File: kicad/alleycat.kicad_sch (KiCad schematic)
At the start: 84 parts, among them U1 E73-2G4M08S1C

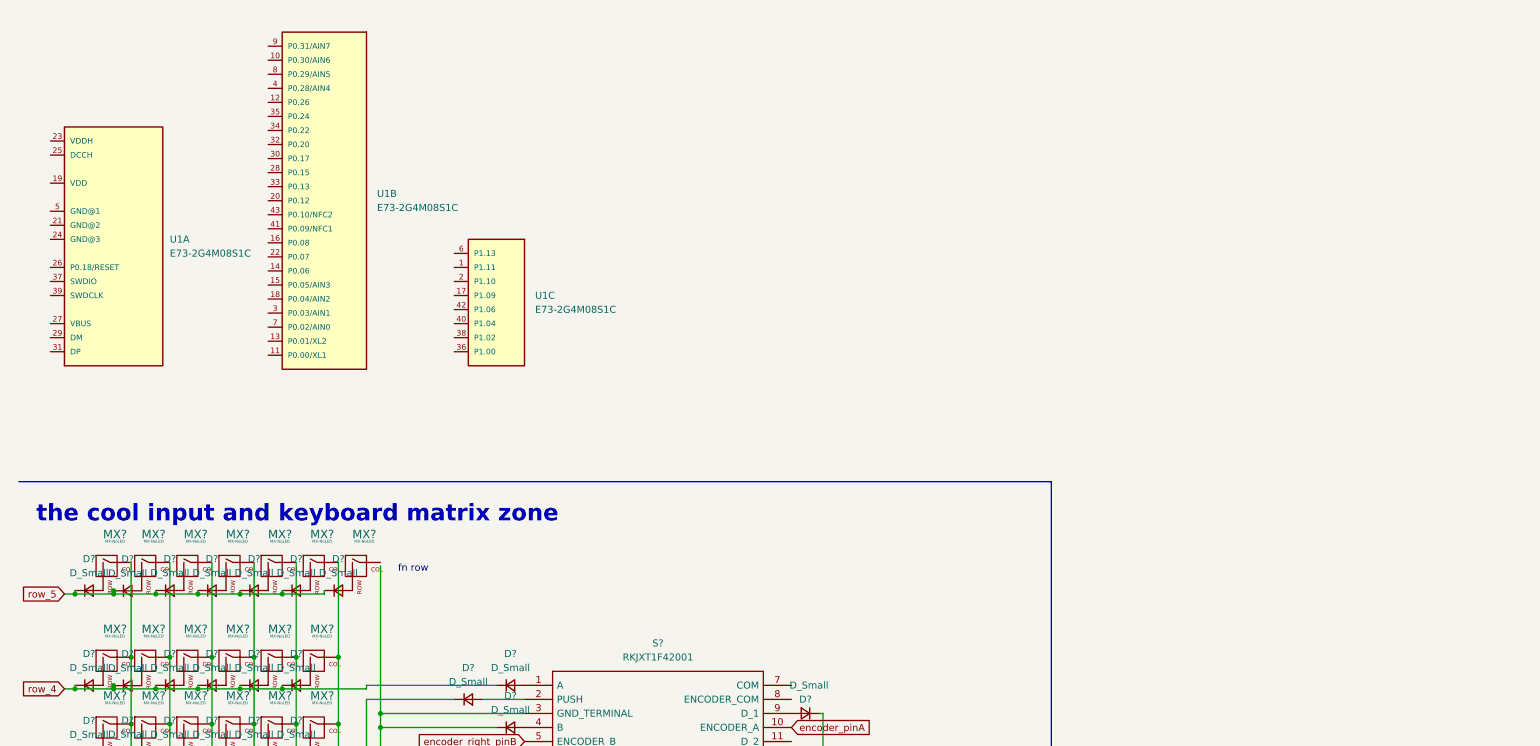
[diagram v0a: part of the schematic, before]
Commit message: nya
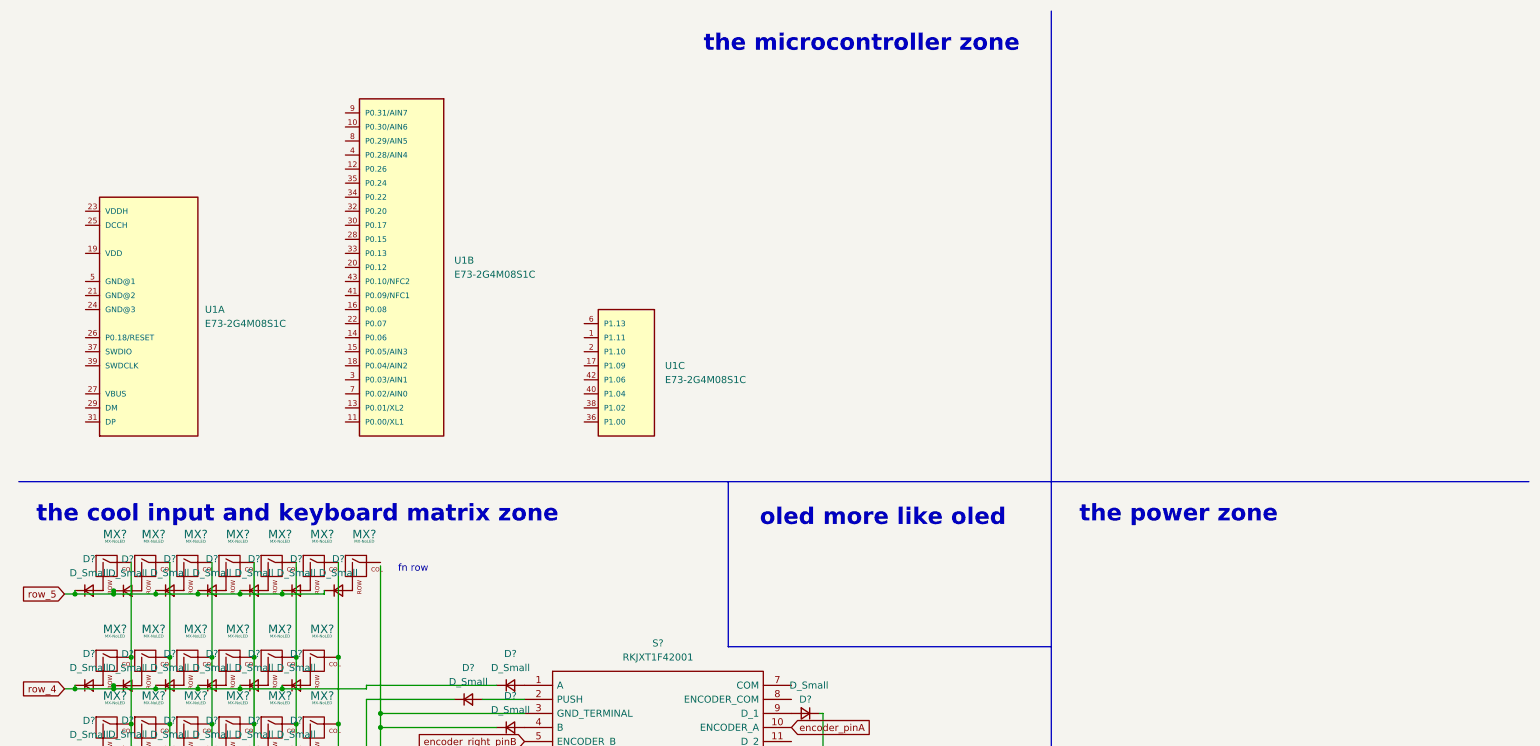
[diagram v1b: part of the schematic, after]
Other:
- note added: "oled more like oled"
- note added: "the microcontroller zone"
- note added: "the power zone"
- moved on the sheet: U1A, U1B, U1C
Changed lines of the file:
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@@
+    (stroke (width 0) (type default) (color 0 0 0 0))
+  )
+  (polyline (pts (xy 140.335 127) (xy 198.755 127))
     (stroke (width 0) (type default) (color 0 0 0 0))
   )
@@
     (stroke (width 0) (type default) (color 0 0 0 0))
   )
+  (polyline (pts (xy 140.335 97.155) (xy 140.335 127))
+    (stroke (width 0) (type default) (color 0 0 0 0))
+  )
   (wire (pts (xy 44.45 146.685) (xy 52.07 146.685))
     (stroke (width 0) (type default) (color 0 0 0 0))
@@
     (stroke (width 0) (type default) (color 0 0 0 0))
   )
+  (polyline (pts (xy 198.755 12.065) (xy 198.755 97.155))
+    (stroke (width 0) (type default) (color 0 0 0 0))
+  )
   (wire (pts (xy 90.805 136.525) (xy 74.93 136.525))
     (stroke (width 0) (type default) (color 0 0 0 0))
@@
   (wire (pts (xy 52.07 184.15) (xy 59.69 184.15))
     (stroke (width 0) (type default) (color 0 0 0 0))
+  )
+  (polyline (pts (xy 198.755 97.155) (xy 285.115 97.155))
+    (stroke (width 0) (type default) (color 0 0 0 0))
+  )
+  (text "the microcontroller zone\n" (at 135.89 19.685 0)
+    (effects (font (size 3 3) bold) (justify left bottom))
   )
   (text "hate that i need another col for one single button"
@@
     (effects (font (size 1.27 1.27)) (justify left bottom))
   )
+  (text "oled more like oled\n" (at 146.05 105.41 0)
+    (effects (font (size 3 3) bold) (justify left bottom))
+  )
   (text "fn row" (at 80.645 113.665 0)
     (effects (font (size 1.27 1.27)) (justify left bottom))
+  )
+  (text "the power zone" (at 203.835 104.775 0)
+    (effects (font (size 3 3) bold) (justify left bottom))
   )
   (text "with the circle pad facing up and flat on the board, pin 4 is left"
@@
     (pin "2")
   )
-  (symbol (lib_id "E73-2G4M08S1C:E73-2G4M08S1C") (at 100.965 66.04 180) (unit 3)
-    (in_bom yes) (on_board yes) (fields_autoplaced)
-    (property "Reference" "U1" (id 0) (at 105.41 63.4999 0)
+  (symbol (lib_id "E73-2G4M08S1C:E73-2G4M08S1C") (at 124.46 78.74 180) (unit 3)
+    (in_bom yes) (on_board yes) (fields_autoplaced)
+    (property "Reference" "U1" (id 0) (at 128.905 76.1999 0)
       (effects (font (size 1.27 1.27)) (justify right))
     )
-    (property "Value" "E73-2G4M08S1C" (id 1) (at 105.41 66.0399 0)
+    (property "Value" "E73-2G4M08S1C" (id 1) (at 128.905 78.7399 0)
       (effects (font (size 1.27 1.27)) (justify right))
     )
-    (property "Footprint" "E73-2G4M08S1C" (id 2) (at 100.965 66.04 0)
+    (property "Footprint" "E73-2G4M08S1C" (id 2) (at 124.46 78.74 0)
       (effects (font (size 1.27 1.27)) (justify left bottom) hide)
     )
-    (property "Datasheet" "" (id 3) (at 100.965 66.04 0)
+    (property "Datasheet" "" (id 3) (at 124.46 78.74 0)
       (effects (font (size 1.27 1.27)) (justify left bottom) hide)
     )
@@
     (pin "2")
   )
-  (symbol (lib_id "E73-2G4M08S1C:E73-2G4M08S1C") (at 69.85 46.355 180) (unit 2)
-    (in_bom yes) (on_board yes) (fields_autoplaced)
-    (property "Reference" "U1" (id 0) (at 76.835 45.0849 0)
+  (symbol (lib_id "E73-2G4M08S1C:E73-2G4M08S1C") (at 83.82 58.42 180) (unit 2)
+    (in_bom yes) (on_board yes) (fields_autoplaced)
+    (property "Reference" "U1" (id 0) (at 90.805 57.1499 0)
       (effects (font (size 1.27 1.27)) (justify right))
     )
-    (property "Value" "E73-2G4M08S1C" (id 1) (at 76.835 47.6249 0)
+    (property "Value" "E73-2G4M08S1C" (id 1) (at 90.805 59.6899 0)
       (effects (font (size 1.27 1.27)) (justify right))
     )
-    (property "Footprint" "E73-2G4M08S1C" (id 2) (at 69.85 46.355 0)
+    (property "Footprint" "E73-2G4M08S1C" (id 2) (at 83.82 58.42 0)
       (effects (font (size 1.27 1.27)) (justify left bottom) hide)
     )
-    (property "Datasheet" "" (id 3) (at 69.85 46.355 0)
+    (property "Datasheet" "" (id 3) (at 83.82 58.42 0)
       (effects (font (size 1.27 1.27)) (justify left bottom) hide)
     )
@@
     (pin "2")
   )
-  (symbol (lib_id "E73-2G4M08S1C:E73-2G4M08S1C") (at 35.56 53.34 0) (unit 1)
-    (in_bom yes) (on_board yes) (fields_autoplaced)
-    (property "Reference" "U1" (id 0) (at 39.37 53.3399 0)
+  (symbol (lib_id "E73-2G4M08S1C:E73-2G4M08S1C") (at 41.91 66.04 0) (unit 1)
+    (in_bom yes) (on_board yes) (fields_autoplaced)
+    (property "Reference" "U1" (id 0) (at 45.72 66.0399 0)
       (effects (font (size 1.27 1.27)) (justify left))
     )
-    (property "Value" "E73-2G4M08S1C" (id 1) (at 39.37 55.8799 0)
+    (property "Value" "E73-2G4M08S1C" (id 1) (at 45.72 68.5799 0)
       (effects (font (size 1.27 1.27)) (justify left))
     )
-    (property "Footprint" "E73-2G4M08S1C" (id 2) (at 35.56 53.34 0)
+    (property "Footprint" "E73-2G4M08S1C" (id 2) (at 41.91 66.04 0)
       (effects (font (size 1.27 1.27)) (justify left bottom) hide)
     )
-    (property "Datasheet" "" (id 3) (at 35.56 53.34 0)
+    (property "Datasheet" "" (id 3) (at 41.91 66.04 0)
       (effects (font (size 1.27 1.27)) (justify left bottom) hide)
     )

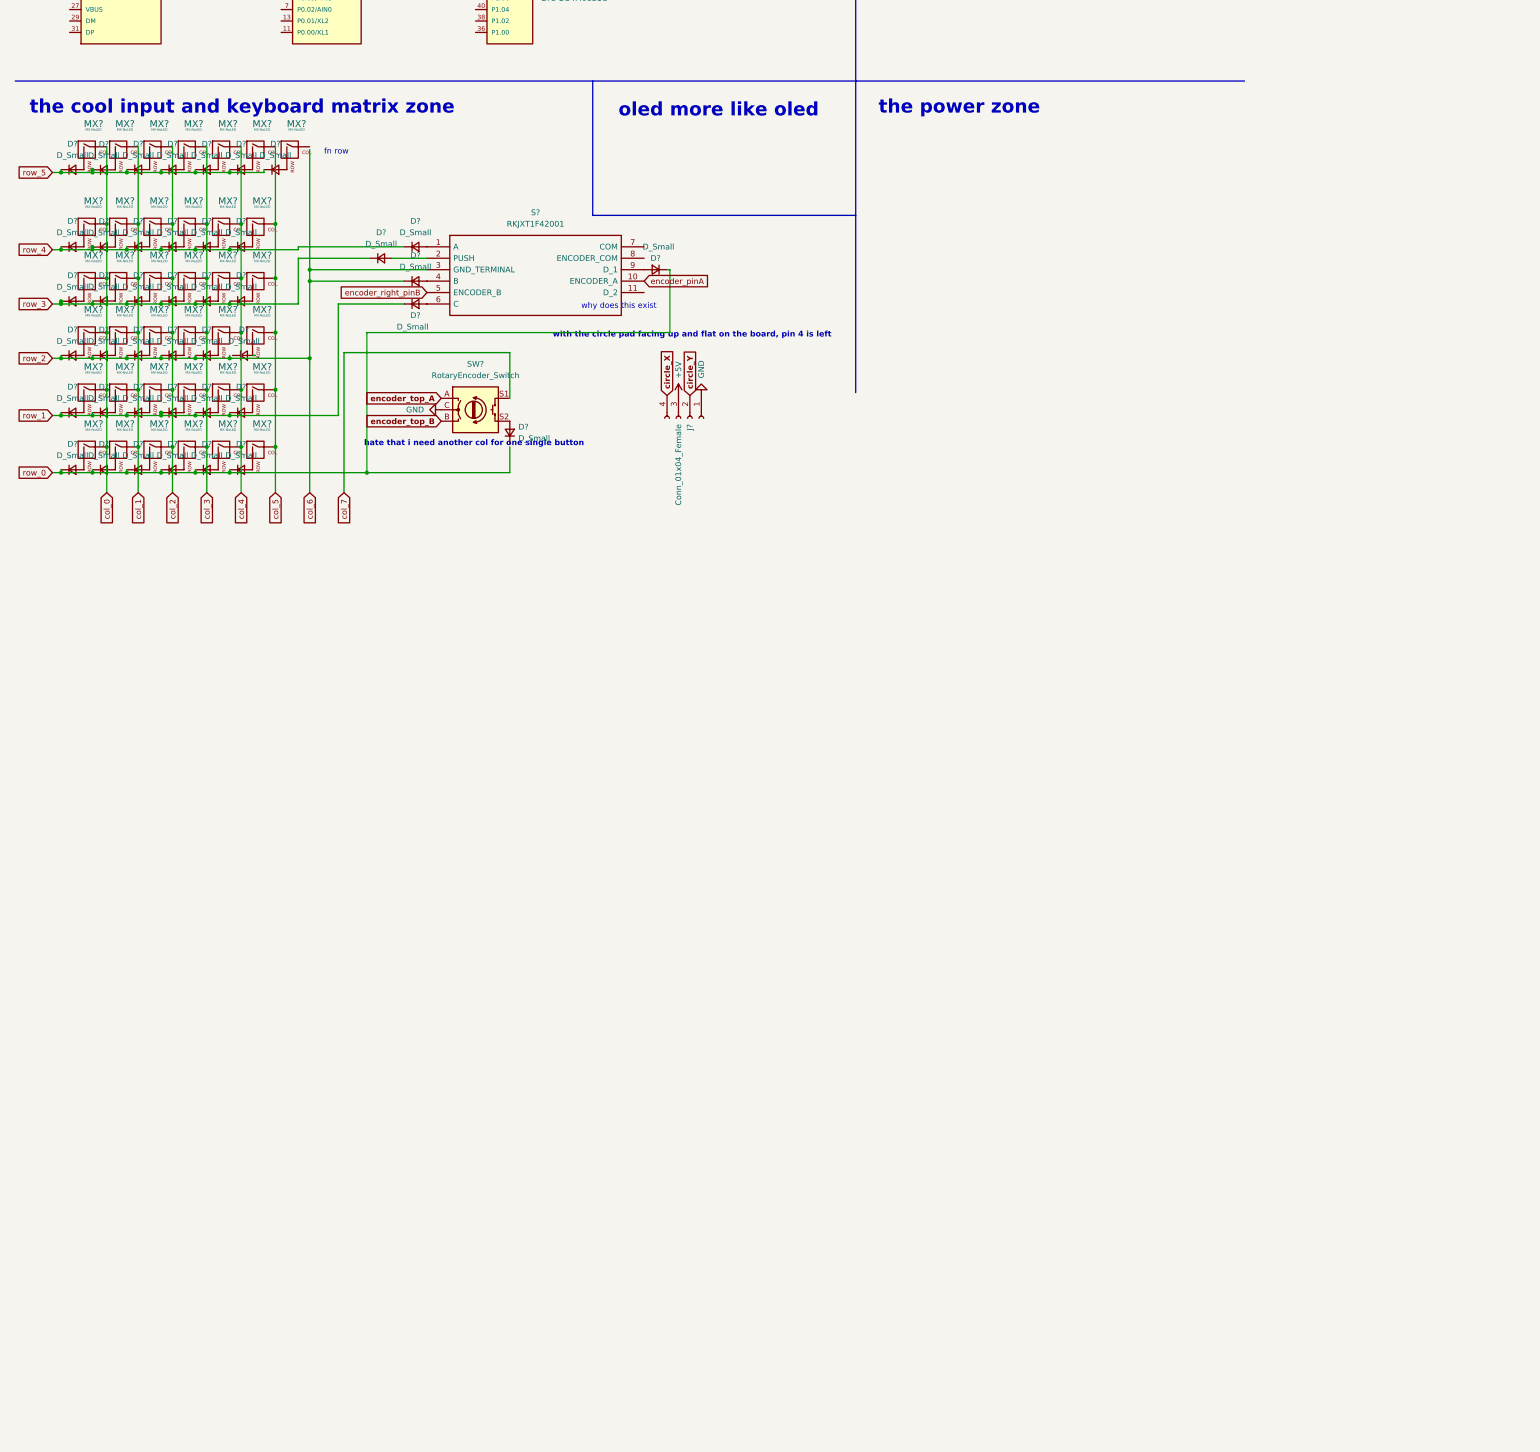
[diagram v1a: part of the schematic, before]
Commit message: cogchamp
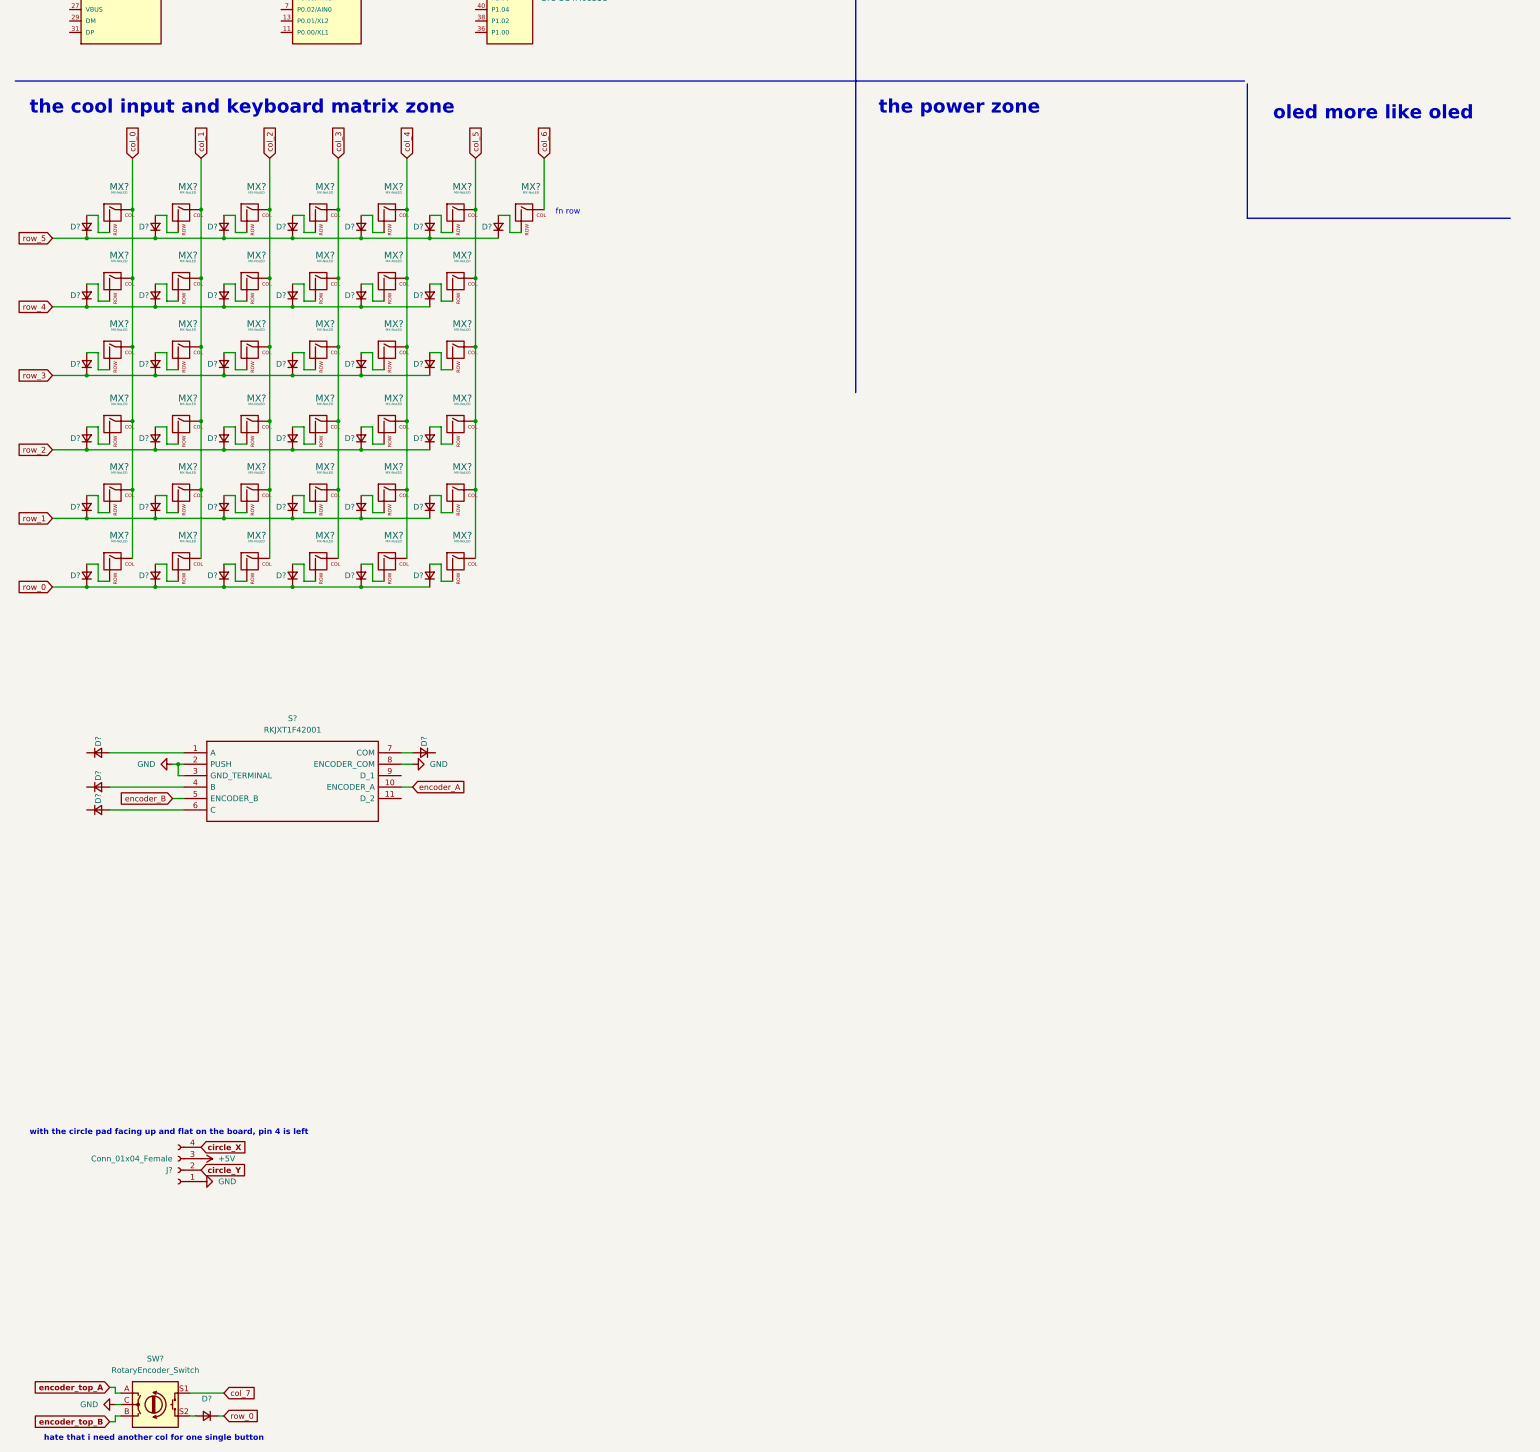
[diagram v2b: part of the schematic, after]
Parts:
- removed D? (x42): D_Small, symbol Device:D_Small
- removed MX? (x36): MX-NoLED, symbol MX_Alps_Hybrid:MX-NoLED
- added D? (x41): D_Small, symbol Device:D_Small
- added MX? (x36): MX-NoLED, symbol MX_Alps_Hybrid:MX-NoLED
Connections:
- net GND: now also S?.2 (PUSH), S?.3 (GND_TERMINAL), S?.8 (ENCODER_COM)
- net col_0: now also MX?.1 (COL), MX?.1 (COL), MX?.1 (COL), MX?.1 (COL), MX?.1 (COL)
- net col_1: now also MX?.1 (COL), MX?.1 (COL), MX?.1 (COL), MX?.1 (COL), MX?.1 (COL), MX?.1 (COL)
- net col_2: now also MX?.1 (COL), MX?.1 (COL), MX?.1 (COL), MX?.1 (COL), MX?.1 (COL), MX?.1 (COL)
- net col_3: now also MX?.1 (COL), MX?.1 (COL), MX?.1 (COL), MX?.1 (COL), MX?.1 (COL), MX?.1 (COL)
- net col_4: now also MX?.1 (COL), MX?.1 (COL), MX?.1 (COL), MX?.1 (COL), MX?.1 (COL), MX?.1 (COL)
- net col_5: now also MX?.1 (COL), MX?.1 (COL), MX?.1 (COL), MX?.1 (COL), MX?.1 (COL), MX?.1 (COL)
- net col_6: now also MX?.1 (COL); no longer S?.3 (GND_TERMINAL)
- net row_0: now also D?.1 (K), D?.1 (K), D?.1 (K), D?.1 (K), D?.1 (K), D?.1 (K), D?.1 (K)
- net row_1: now also D?.1 (K), D?.1 (K), D?.1 (K), D?.1 (K), D?.1 (K), D?.1 (K)
- net row_3: now also D?.1 (K), D?.1 (K), D?.1 (K), D?.1 (K), D?.1 (K), D?.1 (K)
- net row_4: now also D?.1 (K), D?.1 (K), D?.1 (K), D?.1 (K), D?.1 (K), D?.1 (K)
- net row_5: now also D?.1 (K), D?.1 (K), D?.1 (K), D?.1 (K), D?.1 (K), D?.1 (K)
- net at S?.4 (B): now also D?.2 (A)
- net at S?.1 (A): now also D?.2 (A)
- net at S?.6 (C): now also D?.2 (A)
- net at S?.7 (COM): now also D?.2 (A)
- net at SW?.S2: now also D?.2 (A)
- net encoder_pinA renamed encoder_A
- net encoder_right_pinB renamed encoder_B
- new net: D?.2 (A), MX?.2 (ROW) (x36)
- new net row_2: D?.1 (K), D?.1 (K), D?.1 (K), D?.1 (K), D?.1 (K), D?.1 (K)
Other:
- note removed: "why does this exist"
- moved on the sheet: D?, J?, MX?, S?, SW?
